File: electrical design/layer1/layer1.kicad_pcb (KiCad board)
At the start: 2 copper layers, 178 x 158.1 mm, 107 parts, among them J1 SH1.0 Female, J2 SH1.0 5P, J4 Conn_01x03_Female, J5 Conn_01x02_Female, Q1 MOSFET-NCH-FQP30N06L, Q2 MOSFET-NCH-AO3404A, SW1 SW_DPDT_x2, SW2 SW_DPDT_x2, SW3 SW_Push, U1 STM32F103C8T6, U2 CD74HC4067SM, U3 CD74HC4067SM, Y1 Crystal

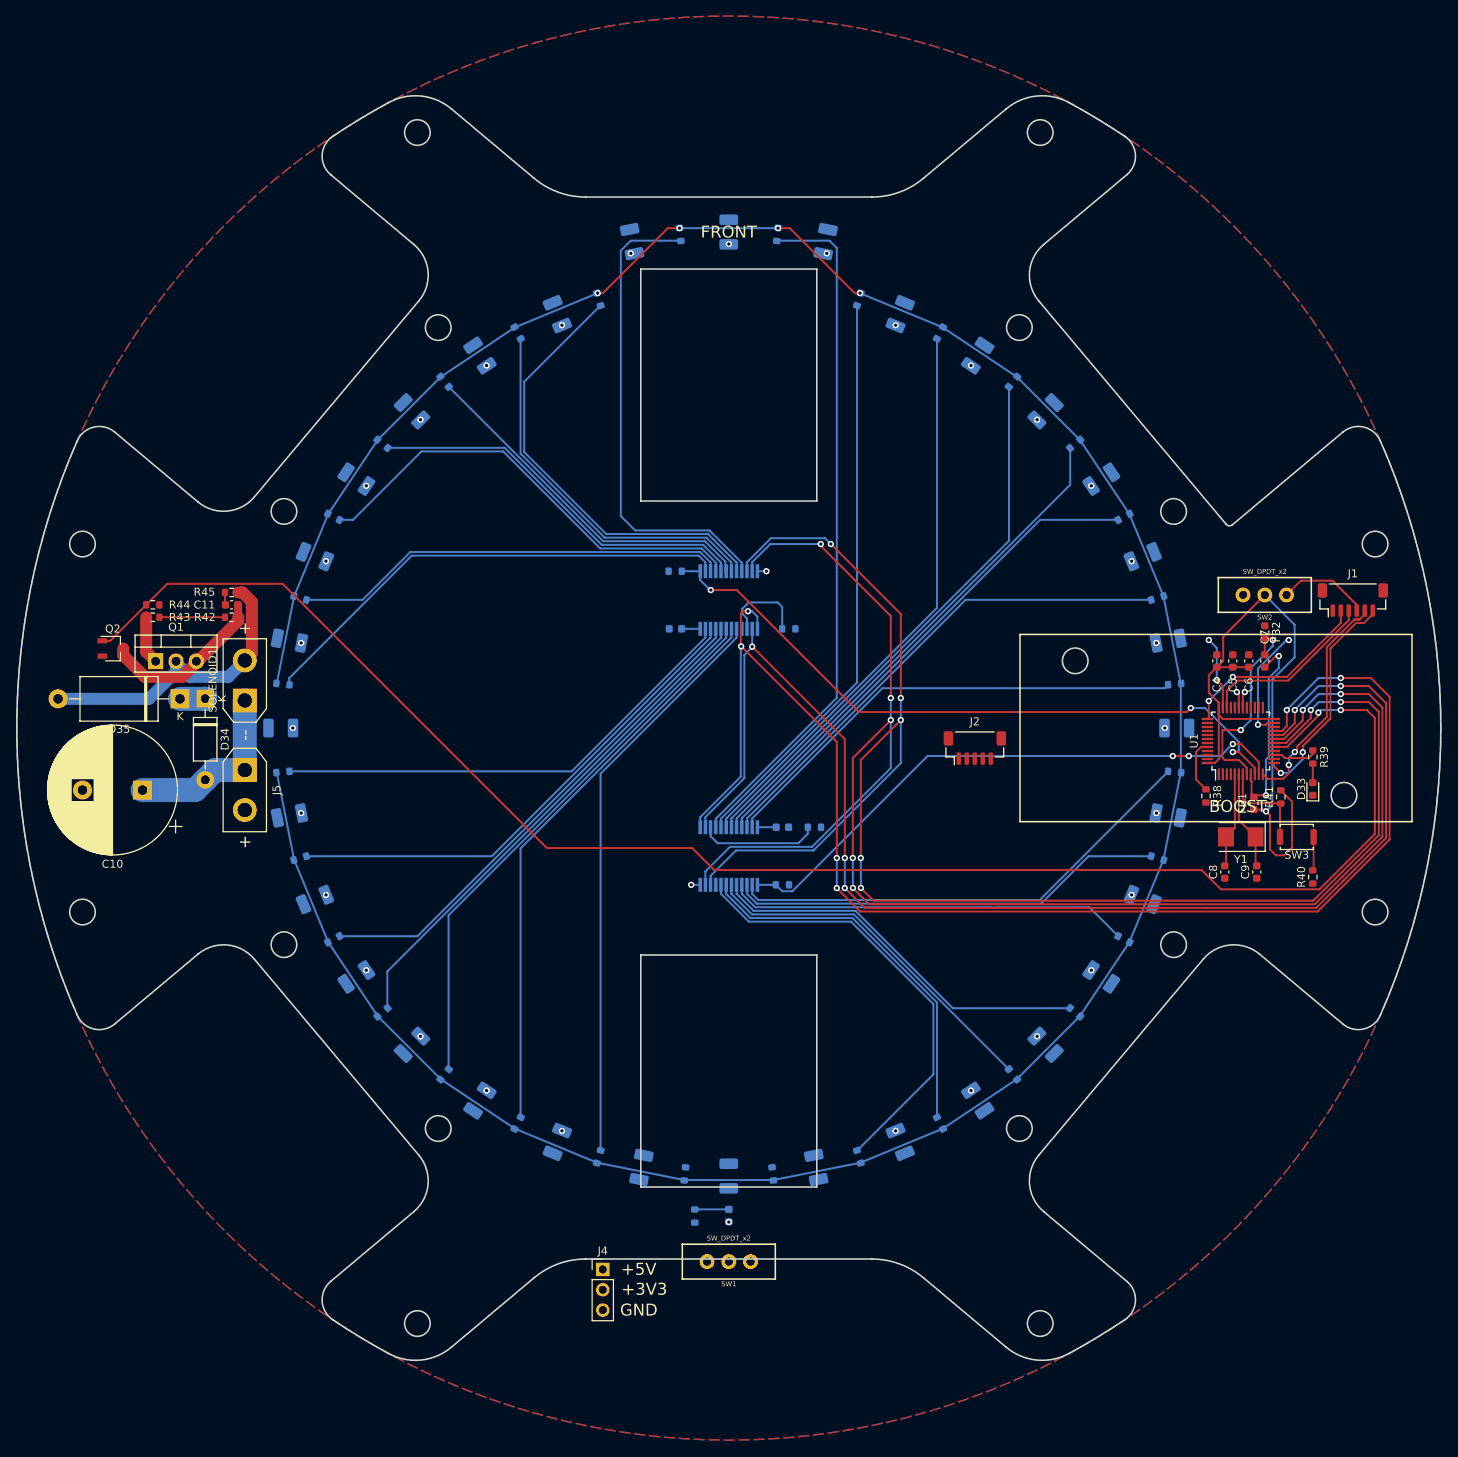
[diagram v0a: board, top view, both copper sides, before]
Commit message: production-ready layer 1!
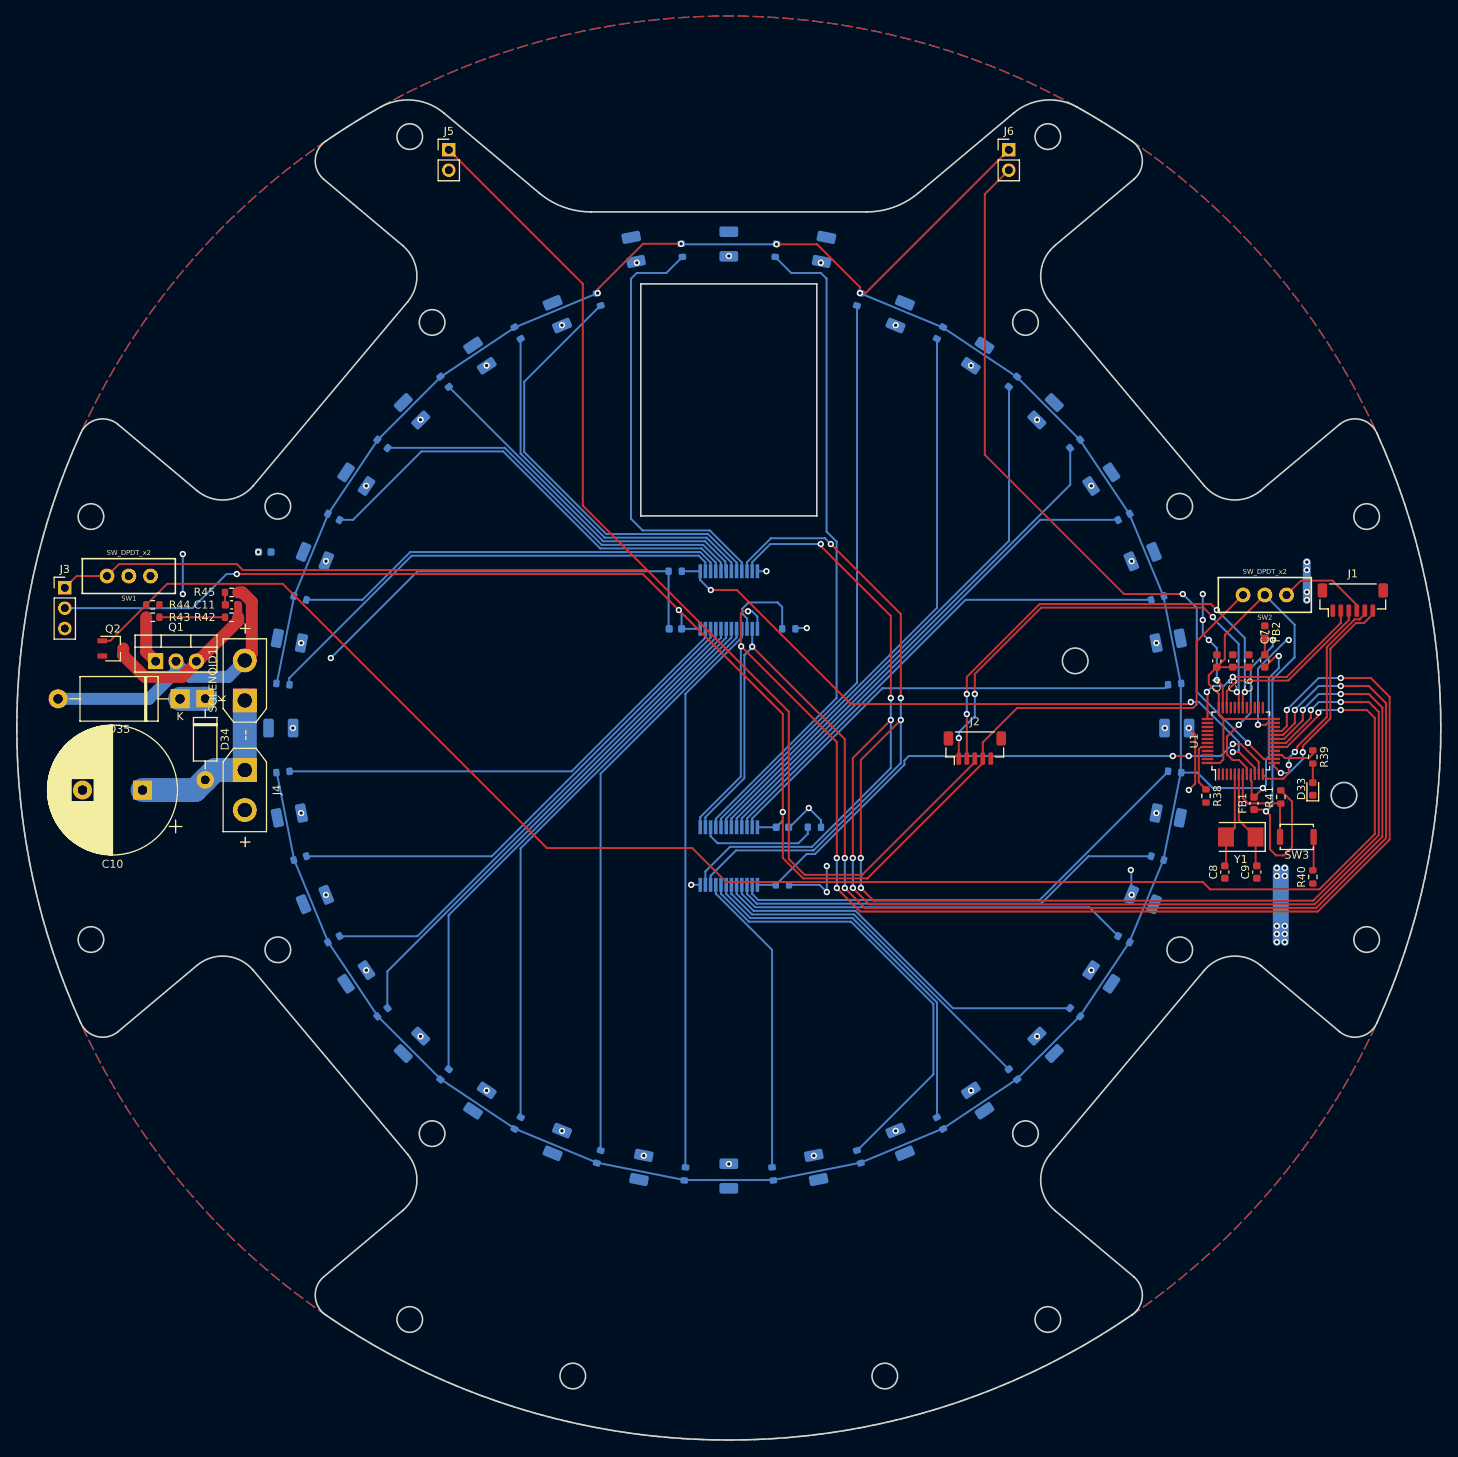
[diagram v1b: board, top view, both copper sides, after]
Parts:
- removed R33: 0.39, Resistor_SMD:R_0603_1608Metric
- added J5: Conn_01x02_Male, Connector_PinHeader_2.54mm:PinHeader_1x02_P2.54mm_Vertical, F.Cu at (75.0, 37.7)
- added J6: Conn_01x02_Male, Connector_PinHeader_2.54mm:PinHeader_1x02_P2.54mm_Vertical, F.Cu at (145.0, 37.7)
- J3: renamed from J4; value Conn_01x03_Female -> DEBUG
- moved SW1 113.9 mm to (35.0, 91.0)
- moved J3 108.5 mm to (27.0, 92.5)
- moved C1 101.2 mm to (52.0, 88.0), turned to 180 degrees
- moved R1 2.00 mm to (104.1, 50.3)
- moved R32 2.00 mm to (115.9, 50.3)
- moved D1 1.50 mm to (110.0, 49.5)
- moved D2 1.00 mm to (98.1, 50.2)
- moved D32 1.00 mm to (121.9, 50.2)
- renumbered J5 to J4
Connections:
- SW1 pad 2: Net-(R33-Pad1) -> Net-(C1-Pad1)
- U1 pad 14: unconnected-(U1-Pad14) -> /LIGHTGATE
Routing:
- net +5V: track 0.00 -> 210.9 mm
- net +3V3: track 4.67 -> 206.1 mm, vias 0 -> 3
- net GND: track 25.9 -> 133.6 mm, vias 36 -> 63
- net /LIGHTGATE: track 0.00 -> 94.9 mm, vias 0 -> 2
- net Net-(R16-Pad2): track 0.00 -> 70.2 mm
- net /TX: track 2.06 -> 59.3 mm, vias 1 -> 4
- net /RX: track 2.06 -> 57.9 mm, vias 1 -> 4
- net Net-(R17-Pad2): track 0.00 -> 38.2 mm
- net VCCQ: track 381.2 -> 416.6 mm
- net Net-(R1-Pad2): track 59.8 -> 54.8 mm
- net Net-(C1-Pad1): track 4.25 -> 8.41 mm, vias 0 -> 2
- net Net-(R32-Pad2): track 86.5 -> 82.9 mm
- net GNDA: track 26.2 -> 23.8 mm
- net /S2: track 170.7 -> 169.7 mm
- net /SWDCLOCK: track 24.4 -> 25.3 mm
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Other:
- board size 178 x 158.1 mm -> 178 x 167.5 mm
- board text removed: "+3V3"
- board text removed: "+5V"
- board text removed: "BOOST"
- board text removed: "FRONT"
- board text removed: "GND"
